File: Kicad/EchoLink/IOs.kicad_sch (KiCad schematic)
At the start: 5 parts, among them J3 Conn_01x08_Pin, J4 Conn_01x06_Pin, J5 Conn_01x09_Socket

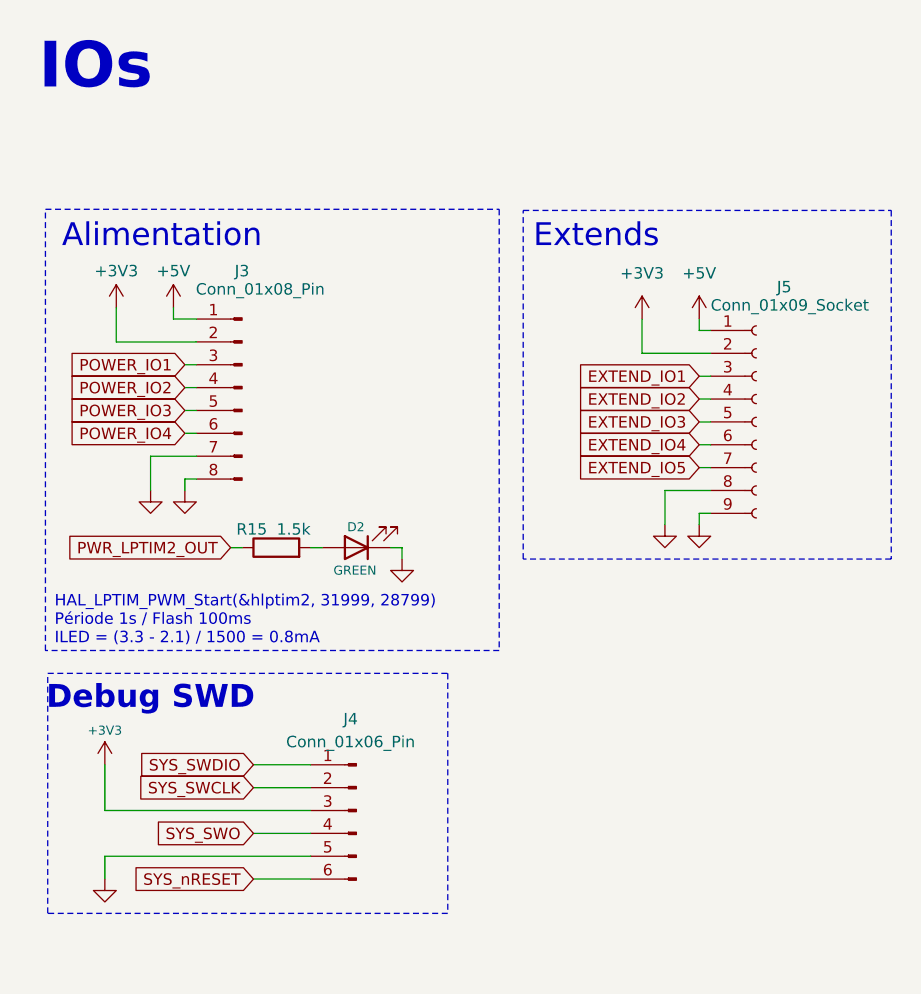
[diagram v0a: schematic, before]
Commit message: wip: add comments in schematic
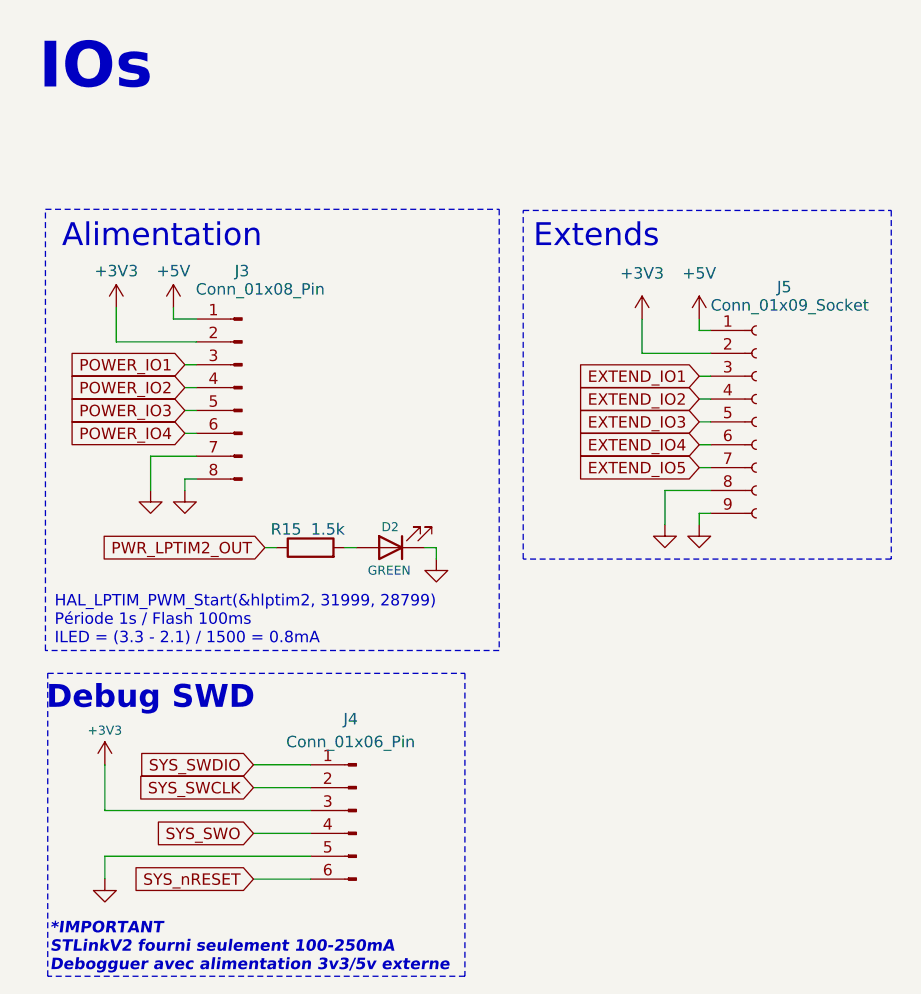
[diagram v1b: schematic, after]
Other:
- note added: "*IMPORTANT STLinkV2 fourni seulement 100-250mA Debogguer avec alimentation 3v3/5v externe"
- moved on the sheet: D2, R15
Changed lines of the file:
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@@
 	(rectangle
 		(start 15.24 85.09)
-		(end 59.69 111.76)
+		(end 61.595 118.745)
 		(stroke
 			(width 0)
@@
 		)
 	)
+	(text "*IMPORTANT\nSTLinkV2 fourni seulement 100-250mA\nDebogguer avec alimentation 3v3/5v externe"
+		(exclude_from_sim no)
+		(at 15.494 115.57 0)
+		(effects
+			(font
+				(size 1.27 1.27)
+				(thickness 0.254)
+				(bold yes)
+				(italic yes)
+			)
+			(justify left)
+		)
+	)
 	(text "HAL_LPTIM_PWM_Start(&hlptim2, 31999, 28799)\nPériode 1s / Flash 100ms\nILED = (3.3 - 2.1) / 1500 = 0.8mA"
 		(exclude_from_sim no)
@@
 	(wire
 		(pts
-			(xy 44.45 71.12) (xy 45.72 71.12)
+			(xy 48.26 71.12) (xy 49.53 71.12)
 		)
 		(stroke
@@
 	(wire
 		(pts
-			(xy 54.61 71.12) (xy 54.61 72.39)
+			(xy 58.42 71.12) (xy 58.42 72.39)
 		)
 		(stroke
@@
 	(wire
 		(pts
-			(xy 35.56 71.12) (xy 36.83 71.12)
-		)
-		(stroke
-			(width 0)
-			(type default)
-		)
-	)
-	(wire
-		(pts
-			(xy 53.34 71.12) (xy 54.61 71.12)
+			(xy 39.37 71.12) (xy 40.64 71.12)
+		)
+		(stroke
+			(width 0)
+			(type default)
+		)
+	)
+	(wire
+		(pts
+			(xy 57.15 71.12) (xy 58.42 71.12)
 		)
 		(stroke
@@
 	(global_label "PWR_LPTIM2_OUT"
 		(shape input)
-		(at 35.56 71.12 180)
+		(at 39.37 71.12 180)
 		(fields_autoplaced yes)
 		(effects
@@
 		)
 		(property "Intersheetrefs" "${INTERSHEET_REFS}"
-			(at 16.4882 71.12 0)
+			(at 20.2982 71.12 0)
 			(hide yes)
 			(show_name no)
@@
 	(symbol
 		(lib_id "Device:LED")
-		(at 49.53 71.12 180)
+		(at 53.34 71.12 180)
 		(unit 1)
 		(body_style 1)
@@
 		(dnp no)
 		(property "Reference" "D2"
-			(at 48.514 68.834 0)
+			(at 52.324 68.834 0)
 			(show_name no)
 			(do_not_autoplace no)
@@
 		)
 		(property "Value" "GREEN"
-			(at 46.99 73.66 0)
+			(at 50.8 73.66 0)
 			(show_name no)
 			(do_not_autoplace no)
@@
 		)
 		(property "Footprint" "ODB:LED_QBLP601-AG15"
-			(at 49.53 71.12 0)
+			(at 53.34 71.12 0)
 			(hide yes)
 			(show_name no)
@@
 		)
 		(property "Datasheet" "https://www.digikey.ca/en/products/detail/qt-brightek-qtb/QBLP601-AG15/16499667"
-			(at 49.53 71.12 0)
+			(at 53.34 71.12 0)
 			(hide yes)
 			(show_name no)
@@
 		)
 		(property "Description" ""
-			(at 49.53 71.12 0)
+			(at 53.34 71.12 0)
 			(hide yes)
 			(show_name no)
@@
 		)
 		(property "DigiKey_Part_Number" "1516-QBLP601-AG15CT-ND"
-			(at 49.53 71.12 0)
+			(at 53.34 71.12 0)
 			(hide yes)
 			(show_name no)
@@
 		)
 		(property "Purchase-URL" ""
-			(at 49.53 71.12 0)
+			(at 53.34 71.12 0)
 			(hide yes)
 			(show_name no)
@@
 		)
 		(property "Sim.Device" ""
-			(at 49.53 71.12 0)
+			(at 53.34 71.12 0)
 			(hide yes)
 			(show_name no)
@@
 		)
 		(property "Sim.Pins" ""
-			(at 49.53 71.12 0)
+			(at 53.34 71.12 0)
 			(hide yes)
 			(show_name no)
@@
 		)
 		(property "Sim.Type" ""
-			(at 49.53 71.12 0)
+			(at 53.34 71.12 0)
 			(hide yes)
 			(show_name no)
@@
 		)
 		(property "Manufacturer_Part_Number" "QBLP601-AG15"
-			(at 49.53 71.12 0)
+			(at 53.34 71.12 0)
 			(hide yes)
 			(show_name no)
@@
 	(symbol
 		(lib_id "power:GND")
-		(at 54.61 72.39 0)
+		(at 58.42 72.39 0)
 		(unit 1)
 		(body_style 1)
@@
 		(fields_autoplaced yes)
 		(property "Reference" "#PWR045"
-			(at 54.61 78.74 0)
+			(at 58.42 78.74 0)
 			(hide yes)
 			(show_name no)
@@
 		)
 		(property "Value" "GND"
-			(at 54.61 77.47 0)
+			(at 58.42 77.47 0)
 			(hide yes)
 			(show_name no)
@@
 		)
 		(property "Footprint" ""
-			(at 54.61 72.39 0)
+			(at 58.42 72.39 0)
 			(hide yes)
 			(show_name no)
@@
 		)
 		(property "Datasheet" ""
-			(at 54.61 72.39 0)
+			(at 58.42 72.39 0)
 			(hide yes)
 			(show_name no)
@@
 		)
 		(property "Description" ""
-			(at 54.61 72.39 0)
+			(at 58.42 72.39 0)
 			(hide yes)
 			(show_name no)
@@
 	(symbol
 		(lib_id "Device:R")
-		(at 40.64 71.12 90)
+		(at 44.45 71.12 90)
 		(unit 1)
 		(body_style 1)
@@
 		(dnp no)
 		(property "Reference" "R15"
-			(at 39.624 69.088 90)
+			(at 43.434 69.088 90)
 			(show_name no)
 			(do_not_autoplace no)
@@
 		)
 		(property "Value" "1.5k"
-			(at 44.45 69.088 90)
+			(at 48.26 69.088 90)
 			(show_name no)
 			(do_not_autoplace no)
@@
 		)
 		(property "Footprint" "Resistor_SMD:R_0603_1608Metric"
-			(at 40.64 72.898 90)
+			(at 44.45 72.898 90)
 			(hide yes)
 			(show_name no)
@@
 		)
 		(property "Datasheet" "https://www.digikey.ca/en/products/detail/panasonic-electronic-components/ERA-3AEB152V/1465858"
-			(at 40.64 71.12 0)
+			(at 44.45 71.12 0)
 			(hide yes)
 			(show_name no)
@@
 		)
 		(property "Description" "Resistor"
-			(at 40.64 71.12 0)
+			(at 44.45 71.12 0)
 			(hide yes)
 			(show_name no)
@@
 		)
 		(property "DigiKey_Part_Number" "P1.5KDBCT-ND"
-			(at 40.64 71.12 90)
+			(at 44.45 71.12 90)
 			(hide yes)
 			(show_name no)
@@
 		)
 		(property "Purchase-URL" ""
-			(at 40.64 71.12 90)
+			(at 44.45 71.12 90)
 			(hide yes)
 			(show_name no)
@@
 		)
 		(property "Sim.Device" ""
-			(at 40.64 71.12 90)
+			(at 44.45 71.12 90)
 			(hide yes)
 			(show_name no)
@@
 		)
 		(property "Sim.Pins" ""
-			(at 40.64 71.12 90)
+			(at 44.45 71.12 90)
 			(hide yes)
 			(show_name no)
@@
 		)
 		(property "Sim.Type" ""
-			(at 40.64 71.12 90)
+			(at 44.45 71.12 90)
 			(hide yes)
 			(show_name no)
@@
 		)
 		(property "Manufacturer_Part_Number" "ERA-3AEB152V"
-			(at 40.64 71.12 90)
-			(hide yes)
-			(show_name no)
+			(at 44.45 71.12 90)
+			(hide yes)
+			(show_name no)
